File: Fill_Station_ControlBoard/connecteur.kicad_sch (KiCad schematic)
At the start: 1 part, among them J2 JTAG

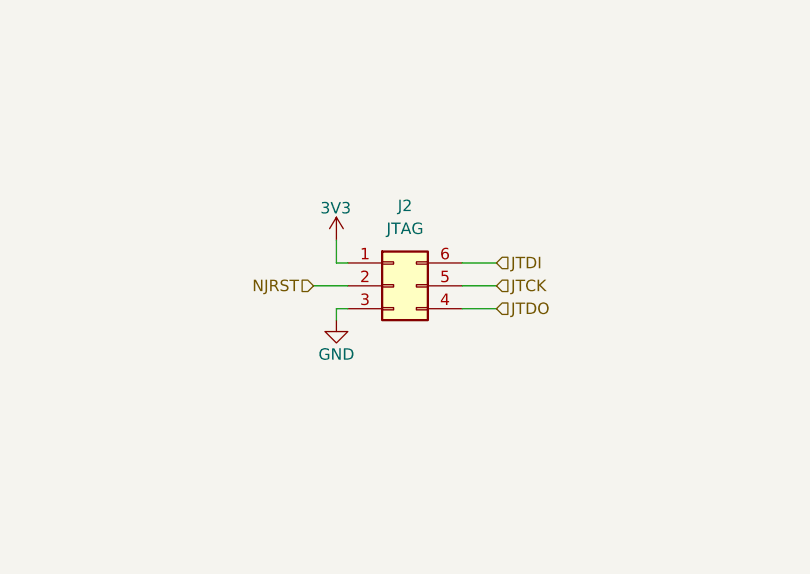
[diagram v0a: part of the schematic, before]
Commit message: Vince
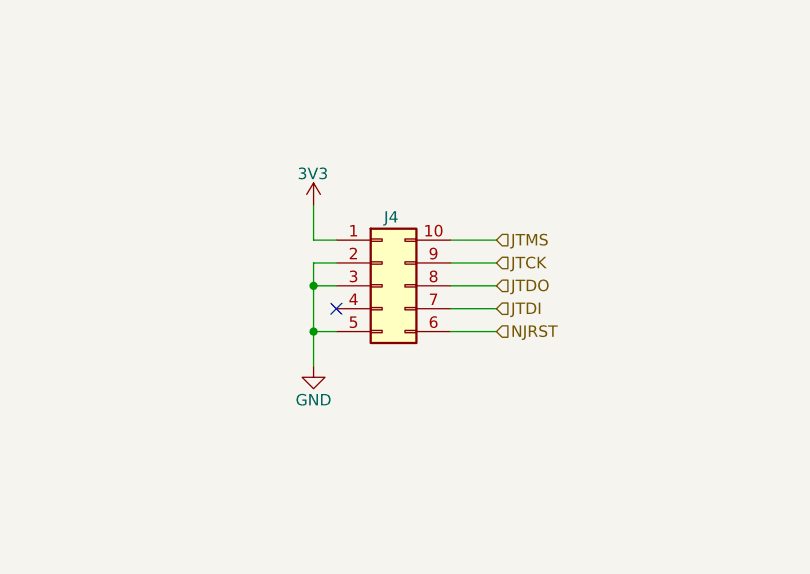
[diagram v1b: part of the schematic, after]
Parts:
- removed J2: JTAG, UserFootprints:490107670612, symbol Connector_Generic:Conn_02x03_Counter_Clockwise
- added J4: Conn_02x05_Counter_Clockwise, symbol Connector_Generic:Conn_02x05_Counter_Clockwise
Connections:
- net 3V3: now also J4.1 (Pin_1)
- net GND: now also J4.2 (Pin_2), J4.3 (Pin_3), J4.5 (Pin_5)
- net JTCK: now also J4.9 (Pin_9)
- net JTDI: now also J4.7 (Pin_7)
- net JTDO: now also J4.8 (Pin_8)
- net NJRST: now also J4.6 (Pin_6)
- new net JTMS: J4.10 (Pin_10)
- no-connect marks 0 -> 1
